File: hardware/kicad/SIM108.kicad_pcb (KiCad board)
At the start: 2 copper layers, 100 x 85 mm, 114 parts, among them J1 Screw_Terminal_01x09, J2 CAN, Q1 BC547, Q10 BC337-40, Q11 BC547, Q12 BC337-40, Q13 BC547, Q14 BC337-40, Q15 BC547, Q16 BC337-40, Q2 BC337-40, Q3 BC547, Q4 BC337-40, Q5 BC547, Q6 BC337-40, Q7 BC547, Q8 BC337-40, Q9 BC547, SW1 PRG, SW2 INSTANCE, SW3 BUS, U1 MCP2551-I-P, U10 SFH617A-1, U11 MAX6816, U12 SFH617A-1, U13 MAX6816, U14 SFH617A-1, U15 MAX6816, U16 SFH617A-1, U17 MAX6816, U18 SFH617A-1, U19 MAX6816, U2 TMR_2411, U20 SFH617A-1, U21 MAX6816, U3 MAX6816, U4 74HC595, U5 Teensy_3.2, U6 SFH617A-1, U7 MAX6816, U8 SFH617A-1, U9 MAX6816

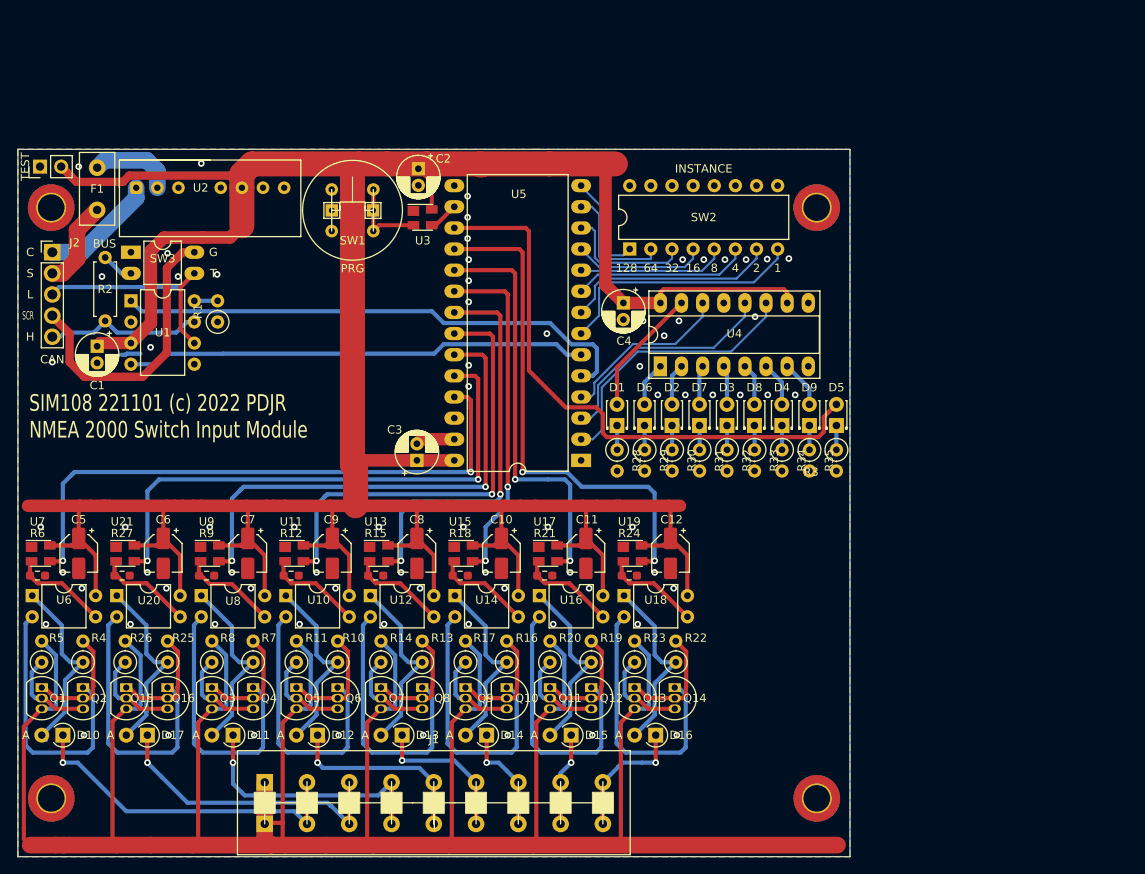
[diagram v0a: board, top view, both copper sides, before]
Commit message: Tweak
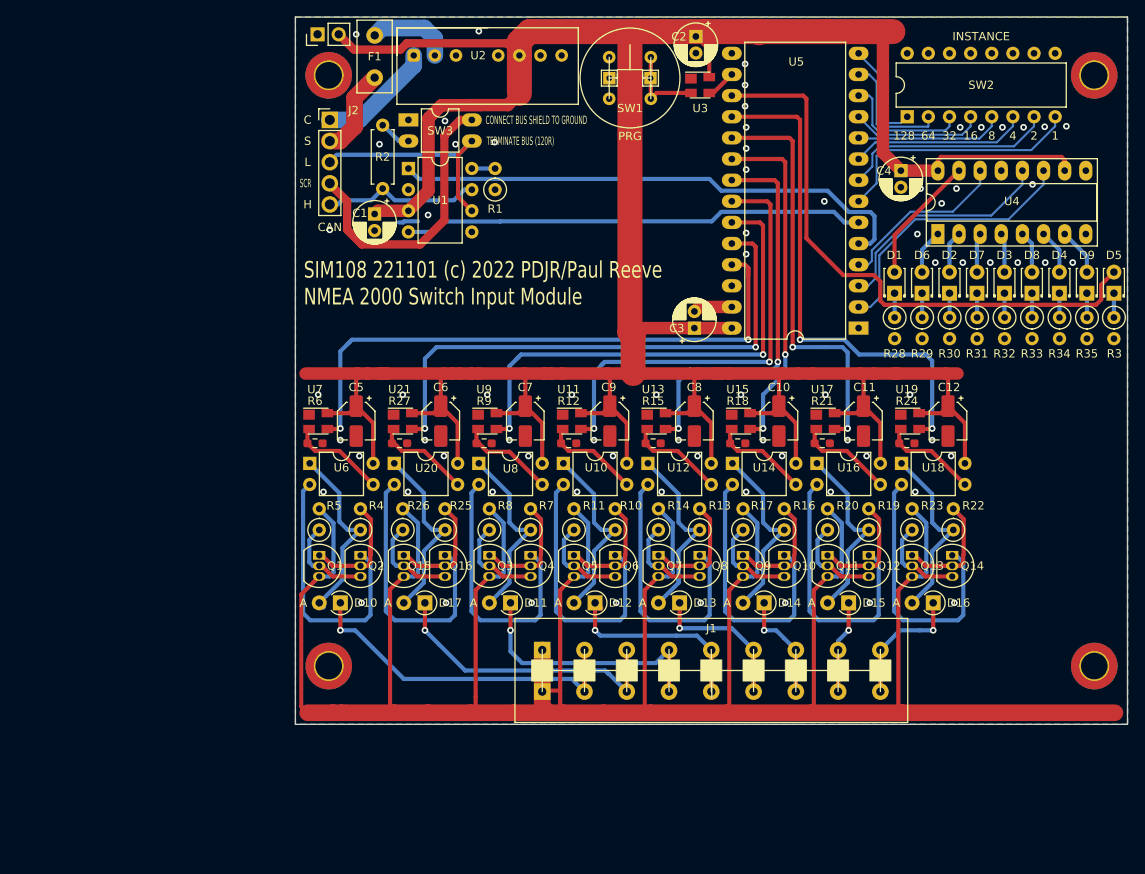
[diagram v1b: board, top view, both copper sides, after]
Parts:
- moved D16 36.9 mm to (96.6, 90.4)
- moved Q12 36.9 mm to (88.9, 84.7)
- moved Q14 36.9 mm to (98.9, 84.7)
- moved Q9 36.9 mm to (73.8, 84.7)
- moved R17 36.9 mm to (73.8, 81.6)
- moved R19 36.9 mm to (88.9, 81.6)
- moved R22 36.9 mm to (99.1, 81.6)
- moved C1 36.9 mm to (29.5, 43.7)
- moved D10 36.9 mm to (25.4, 90.4)
- moved D11 36.9 mm to (45.8, 90.4)
- moved D13 36.9 mm to (66.2, 90.4)
- moved D14 36.9 mm to (76.3, 90.4)
- moved D17 36.9 mm to (35.6, 90.4)
- moved D4 36.9 mm to (111.8, 53.2)
- moved D5 36.9 mm to (118.4, 53.2)
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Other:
- board text added: "CONNECT BUS SHIELD TO GROUND"
- board text added: "SIM108 221101 (c) 2022 PDJR/Paul Reeve NMEA 2000 Switch Input Module"
- board text added: "TERMINATE BUS (120R)"
- board text removed: "G"
- board text removed: "SIM108 221101 (c) 2022 PDJR NMEA 2000 Switch Input Module"
- board text removed: "T"
